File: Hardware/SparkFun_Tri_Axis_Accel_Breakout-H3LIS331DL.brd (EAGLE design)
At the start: 20.3 x 20.3 mm, 23 parts, among them U1 H3LIS331DL

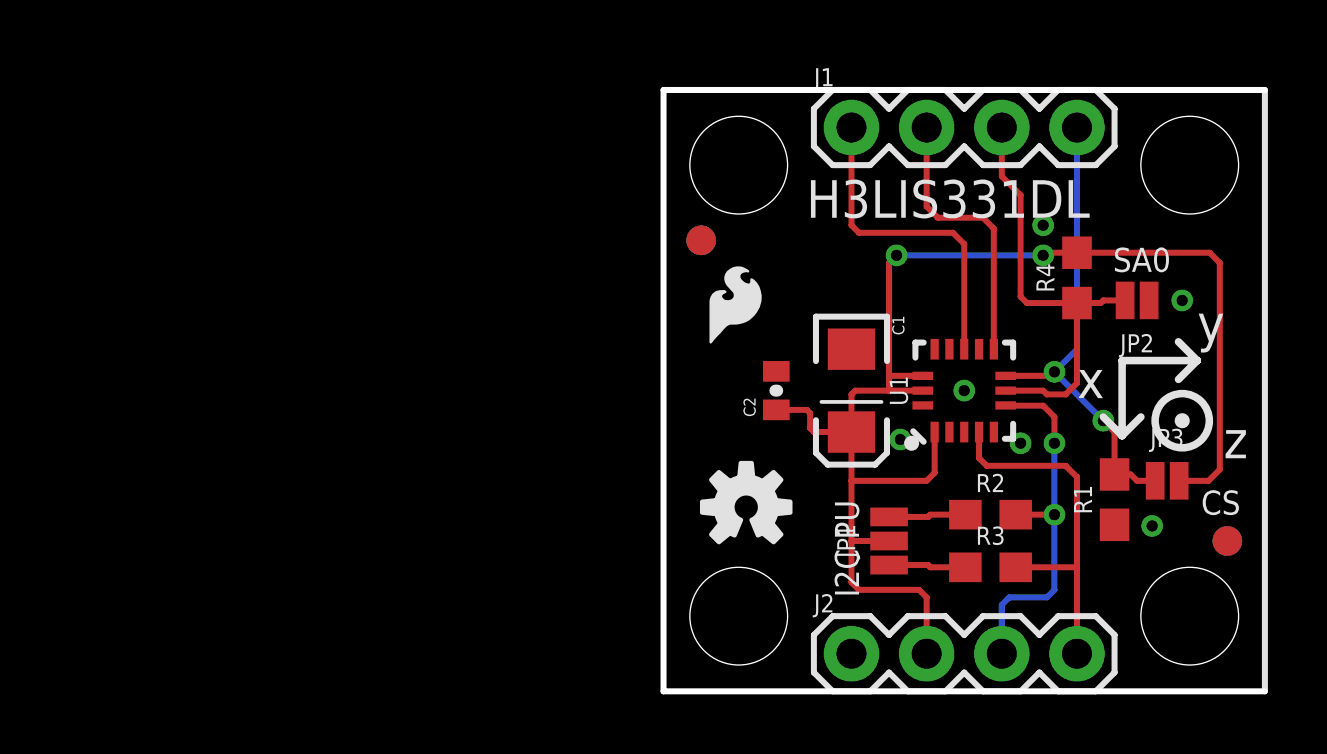
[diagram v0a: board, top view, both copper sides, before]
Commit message: Aesthetic touch ups before review
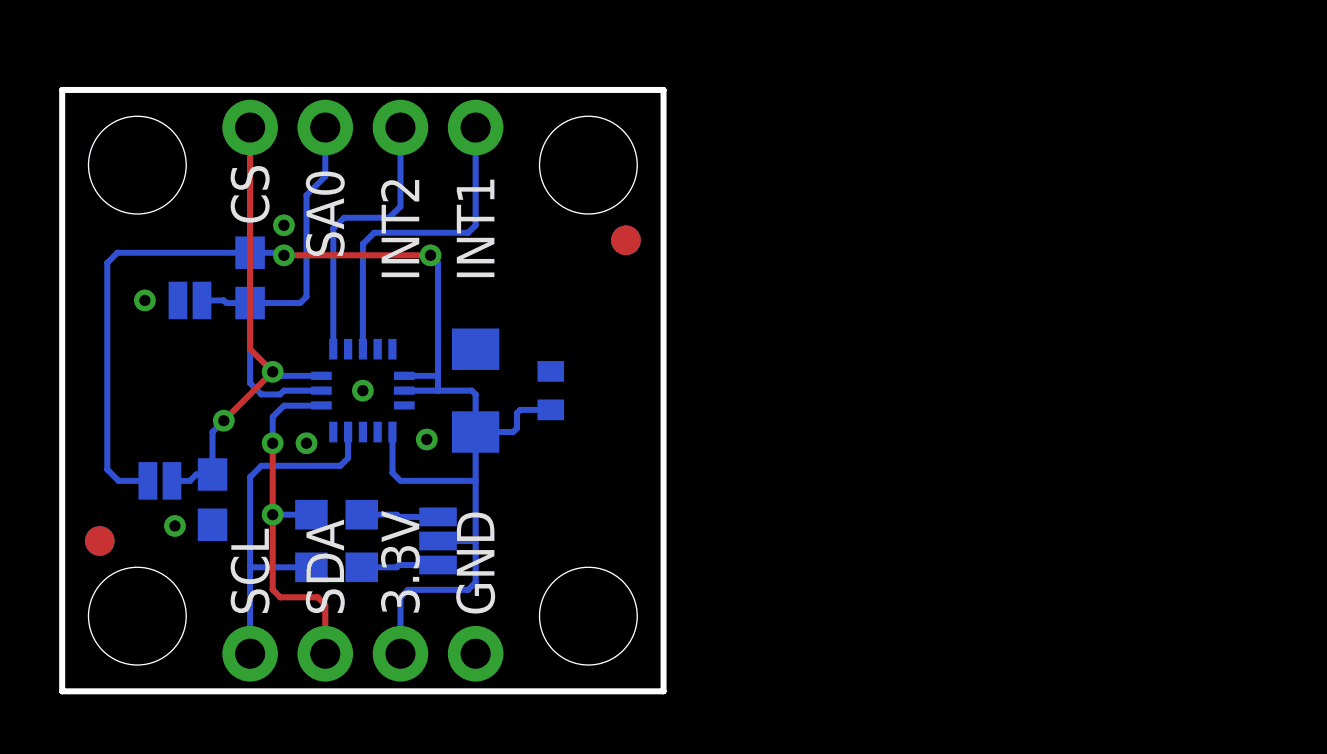
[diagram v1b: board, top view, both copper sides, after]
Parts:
- moved JP6 38.1 mm to (-19.1, 5.08), flipped to the bottom
- moved JP7 38.1 mm to (-19.1, 5.08), flipped to the top
- moved JP10 35.6 mm to (-17.8, 17.8), flipped to the bottom
- moved JP8 35.6 mm to (-17.8, 2.54), flipped to the bottom
- moved JP3 34.0 mm to (-17.0, 7.11), flipped to the bottom
- moved JP2 32.0 mm to (-16.0, 13.2), flipped to the bottom
- moved R1 30.5 mm to (-15.2, 6.48), flipped to the bottom
- moved R4 27.9 mm to (-14.0, 14.0), flipped to the bottom
- moved R2 22.1 mm to (-11.0, 5.97), flipped to the bottom
- moved R3 22.1 mm to (-11.0, 4.19), flipped to the bottom
- moved U1 20.3 mm to (-10.2, 10.2), flipped to the bottom
- moved JP1 15.2 mm to (-7.62, 5.08), flipped to the bottom
- moved C1 12.7 mm to (-6.35, 10.2), flipped to the bottom
- moved J1 12.7 mm to (-6.35, 19.1), flipped to the bottom
- moved J2 12.7 mm to (-6.35, 1.27), flipped to the bottom
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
